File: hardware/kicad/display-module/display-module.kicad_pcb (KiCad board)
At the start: 2 copper layers, 8 parts, among them J1 Exp0, U1 74LS00, U2 74LS373

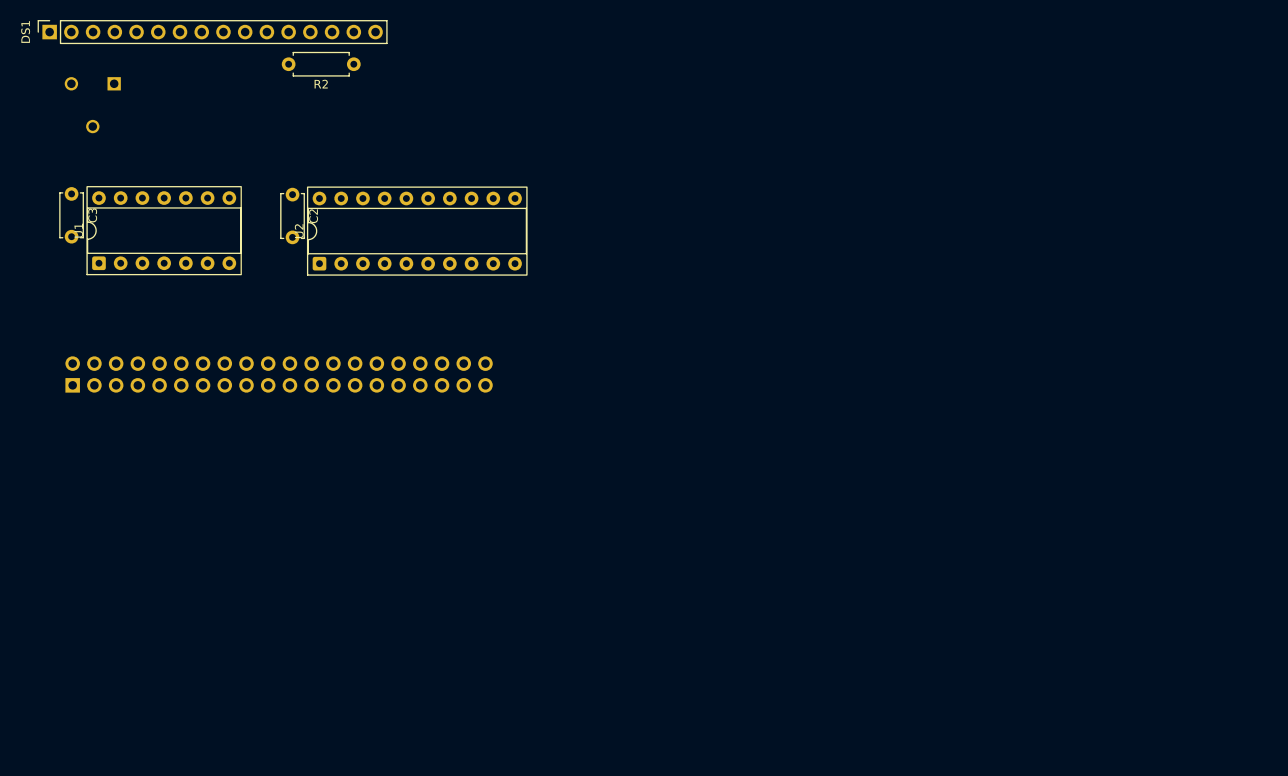
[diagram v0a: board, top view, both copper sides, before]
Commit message: Add mainboard v2.0
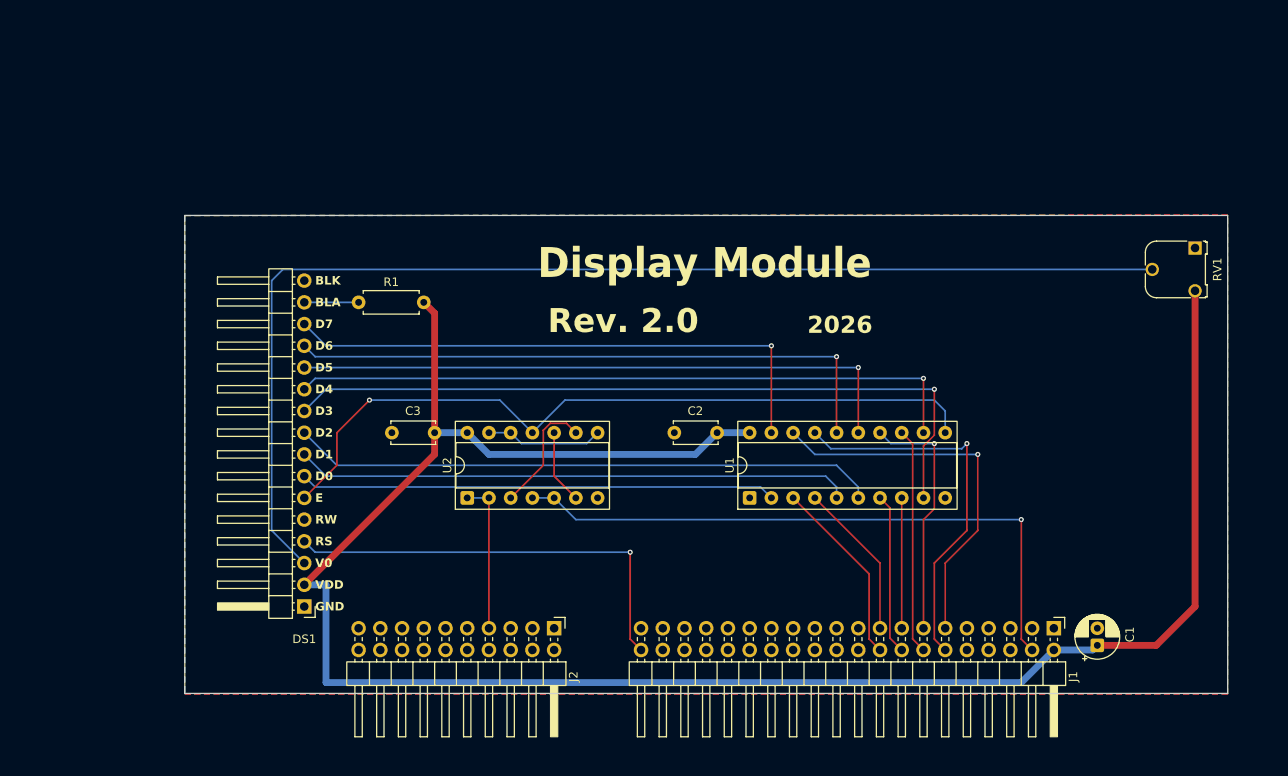
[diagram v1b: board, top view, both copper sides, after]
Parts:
- added C1: 220 uF, Capacitor_THT:CP_Radial_D5.0mm_P2.00mm, F.Cu at (193.0, 113.8)
- added J2: EXP_0_B, Connector_PinHeader_2.54mm:PinHeader_2x10_P2.54mm_Horizontal, F.Cu at (129.5, 111.8)
- DS1: value WC1602A -> WC1604A; footprint Connector_PinSocket_2.54mm:PinSocket_1x16_P2.54mm_Vertical -> Connector_PinHeader_2.54mm:PinHeader_1x16_P2.54mm_Horizontal
- J1: value Exp0 -> EXP_0_A; footprint Connector_PinSocket_2.54mm:PinSocket_2x20_P2.54mm_Vertical -> Connector_PinHeader_2.54mm:PinHeader_2x20_P2.54mm_Horizontal; moved to F.Cu
- RV1: moved to F.Cu
- moved RV1 127.8 mm to (204.5, 67.3), turned to -90 degrees
- moved J1 118.2 mm to (188.0, 111.8)
- moved DS1 73.5 mm to (100.3, 109.2), turned to 180 degrees
- moved U1 57.3 mm to (152.4, 96.5)
- moved C2 56.9 mm to (148.6, 88.9), turned to 180 degrees
- moved U2 51.0 mm to (119.4, 96.5)
- moved C3 50.8 mm to (115.6, 88.9), turned to 180 degrees
- moved R1 27.8 mm to (106.7, 73.7), turned to 0 degrees
- renumbered R2 to R1, U2 to U1, U1 to U2
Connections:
- J1 pad 10: /A12 -> GND
- J1 pad 11: /A11 -> /D7
- J1 pad 12: /A10 -> /D6
- J1 pad 13: /A9 -> /D5
- J1 pad 14: /A8 -> /D4
- J1 pad 15: /A7 -> /D3
- J1 pad 16: /A6 -> /D2
- J1 pad 17: /A5 -> /D1
- J1 pad 18: /A4 -> /D0
- J1 pad 19: /A3 -> GND
- J1 pad 20: /A2 -> GND
- J1 pad 21: /A1 -> /A19
- J1 pad 22: /A0 -> /A18
- J1 pad 23: /D7 -> /A17
- J1 pad 24: /D6 -> /A16
- J1 pad 25: /D5 -> /A15
- J1 pad 26: /D4 -> /A14
- J1 pad 27: /D3 -> /A13
- J1 pad 28: /D2 -> /A12
- J1 pad 29: /D1 -> /A11
- J1 pad 3: /A19 -> /IOM
- J1 pad 30: /D0 -> /A10
- J1 pad 31: /IOM -> /A9
- J1 pad 32: /RD -> /A8
- J1 pad 33: /WR -> /A7
- J1 pad 34: /RDY -> /A6
- J1 pad 35: /RESET -> /A5
- J1 pad 36: /ALE -> /A4
- J1 pad 37: /MEM_EXP0_CS -> /A3
- J1 pad 38: /IO_EXP_CS -> /A2
- J1 pad 39: GND -> /A1
- J1 pad 4: /A18 -> /WR
- J1 pad 40: /CLK -> /A0
- J1 pad 5: /A17 -> /RD
- J1 pad 6: /A16 -> /RDY
- J1 pad 7: /A15 -> /RESET
- J1 pad 8: /A14 -> /NMI
- J1 pad 9: /A13 -> /ALE
- U2 pad 1: /IO_EXP_CS -> /EXP_IO_CS4
- U2 pad 2: /IO_EXP_CS -> /EXP_IO_CS4
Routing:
- net VCC: track 0.00 -> 235.0 mm
- net Net-(DS1-VO): track 0.00 -> 138.1 mm
- net /LCD_WRITE: track 0.00 -> 88.1 mm, vias 0 -> 1
- net Net-(DS1-D3): track 0.00 -> 87.9 mm, vias 0 -> 1
- net Net-(DS1-D4): track 0.00 -> 79.3 mm, vias 0 -> 1
- net /WR: track 0.00 -> 74.0 mm, vias 0 -> 1
- net Net-(DS1-D5): track 0.00 -> 72.4 mm, vias 0 -> 1
- net Net-(DS1-D6): track 0.00 -> 71.6 mm, vias 0 -> 1
- net Net-(DS1-D2): track 0.00 -> 68.7 mm
- net Net-(DS1-D7): track 0.00 -> 65.8 mm, vias 0 -> 1
- net Net-(DS1-D1): track 0.00 -> 65.1 mm
- net Net-(DS1-D0): track 0.00 -> 55.7 mm
- net /A0: track 0.00 -> 50.6 mm, vias 0 -> 1
- net /D6: track 0.00 -> 45.0 mm, vias 0 -> 1
- net /D7: track 0.00 -> 44.5 mm, vias 0 -> 1
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- added copper zone on B.Cu, net GND
- added copper zone on F.Cu, net GND
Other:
- board outline added: 121.9 x 55.9 mm
- board text added: "2026"
- board text added: "BLA"
- board text added: "BLK"
- board text added: "D0"
- board text added: "D1"
- board text added: "D2"
- board text added: "D3"
- board text added: "D4"
- board text added: "D5"
- board text added: "D6"
- board text added: "D7"
- board text added: "Display Module"
- board text added: "E"
- board text added: "GND"
- board text added: "RS"
- board text added: "RW"
- board text added: "Rev. 2.0"
- board text added: "V0"
- board text added: "VDD"

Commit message: Update mainboard and expansion modules
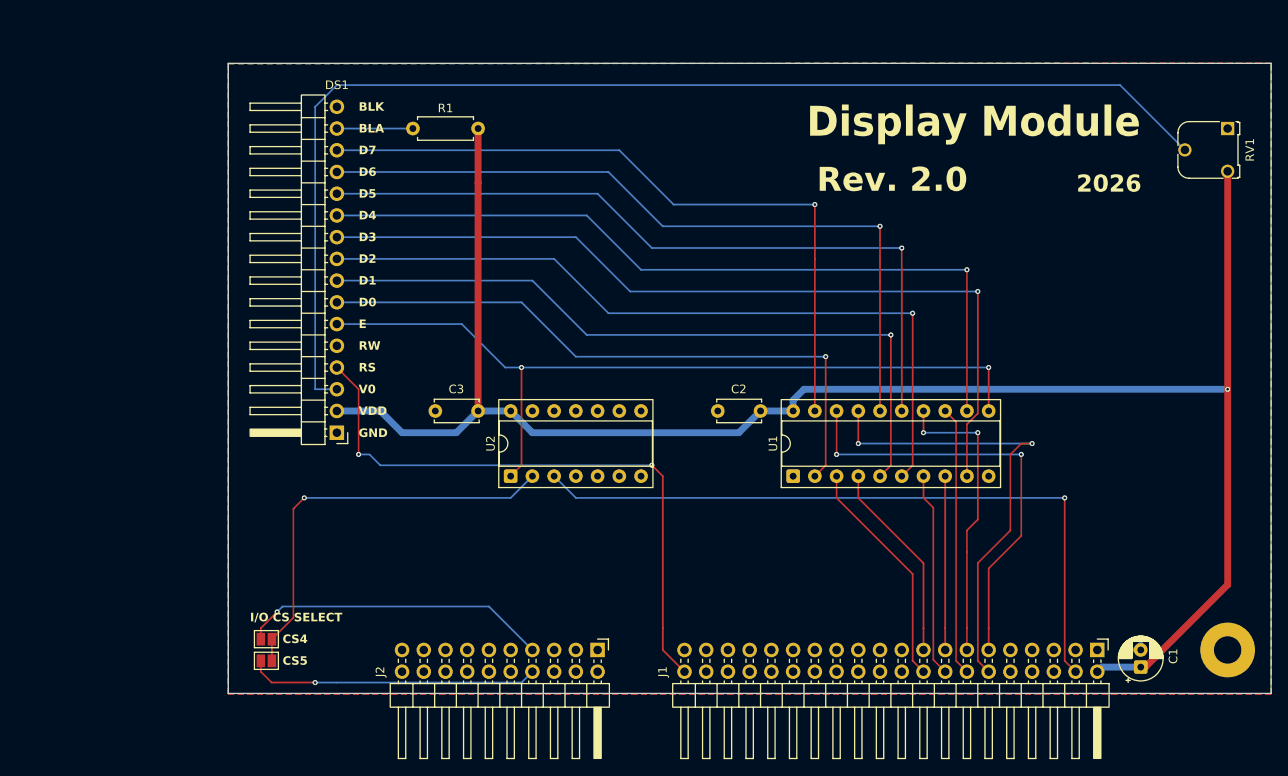
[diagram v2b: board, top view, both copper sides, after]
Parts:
- added H1: MountingHole_Pad, MountingHole:MountingHole_3.2mm_M3_Pad, F.Cu at (208.3, 114.3)
- added JP1: Jumper_2_Small_Open, Jumper:SolderJumper-2_P1.3mm_Open_Pad1.0x1.5mm, F.Cu at (95.9, 113.0)
- added JP2: Jumper_2_Small_Open, Jumper:SolderJumper-2_P1.3mm_Open_Pad1.0x1.5mm, F.Cu at (95.9, 115.6)
- U2: value 74LS00 -> 74LS02
- moved R1 21.3 mm to (113.0, 53.3)
- moved DS1 20.7 mm to (104.1, 88.9)
- moved RV1 14.5 mm to (208.3, 53.3)
- moved C2 5.68 mm to (153.7, 86.4)
- moved U1 5.68 mm to (157.5, 94.0)
- moved C3 5.68 mm to (120.7, 86.4)
- moved C1 5.68 mm to (198.1, 116.3)
- moved J2 5.68 mm to (134.6, 114.3)
- moved U2 5.68 mm to (124.5, 94.0)
- moved J1 5.68 mm to (193.0, 114.3)
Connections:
- U2 pad 1: /EXP_IO_CS4 -> /LCD_WRITE
- U2 pad 10: /WR_N -> unconnected-(U2-Pad10)
- U2 pad 11: /LCD_WRITE -> GND
- U2 pad 12: Net-(U2-Pad12) -> GND
- U2 pad 13: Net-(U2-Pad12) -> unconnected-(U2-Pad13)
- U2 pad 2: /EXP_IO_CS4 -> /DISPLAY_IO_CS
- U2 pad 3: /CS_N -> /WR
- U2 pad 4: /WR -> unconnected-(U2-Pad4)
- U2 pad 5: /WR -> GND
- U2 pad 6: /WR_N -> GND
- U2 pad 8: Net-(U2-Pad12) -> GND
- U2 pad 9: /CS_N -> GND
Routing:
- net /DISPLAY_IO_CS: track 0.00 -> 48.3 mm, vias 0 -> 1
- net /EXP_IO_CS5: track 0.00 -> 34.1 mm, vias 0 -> 1
- net VCC: track 235.0 -> 211.0 mm, vias 0 -> 1
- net /A0: track 50.6 -> 71.7 mm, vias 1 -> 2
- net Net-(DS1-D2): track 68.7 -> 89.5 mm, vias 0 -> 1
- net Net-(DS1-D1): track 65.1 -> 84.4 mm, vias 0 -> 1
- net Net-(DS1-D0): track 55.7 -> 74.3 mm, vias 0 -> 1
- net /EXP_IO_CS4: track 17.8 -> 36.2 mm, vias 0 -> 1
- net Net-(DS1-D7): track 65.8 -> 82.6 mm
- net Net-(DS1-D6): track 71.6 -> 87.7 mm
- net Net-(DS1-D5): track 72.4 -> 87.7 mm
- net /CS_N: track 14.1 -> 0.00 mm
- net Net-(U2-Pad12): track 13.8 -> 0.00 mm
- net Net-(DS1-D4): track 79.3 -> 92.8 mm
- net Net-(DS1-D3): track 87.9 -> 99.7 mm
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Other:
- board size 121.9 x 55.9 mm -> 121.9 x 73.7 mm
- board text added: "CS4"
- board text added: "CS5"
- board text added: "I/O CS SELECT"
